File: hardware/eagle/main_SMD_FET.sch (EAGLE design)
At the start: 44 parts, among them IC1 R-78E3.3-1.0, IC2 INA186A1QDCKRQ1, IC3 ESP-12E/F, J4 1727078, Q1 IRFU3710ZPBF, Q2 IRFU3710ZPBF, Q3 IRFU3710ZPBF, Q4 IRFU3710ZPBF

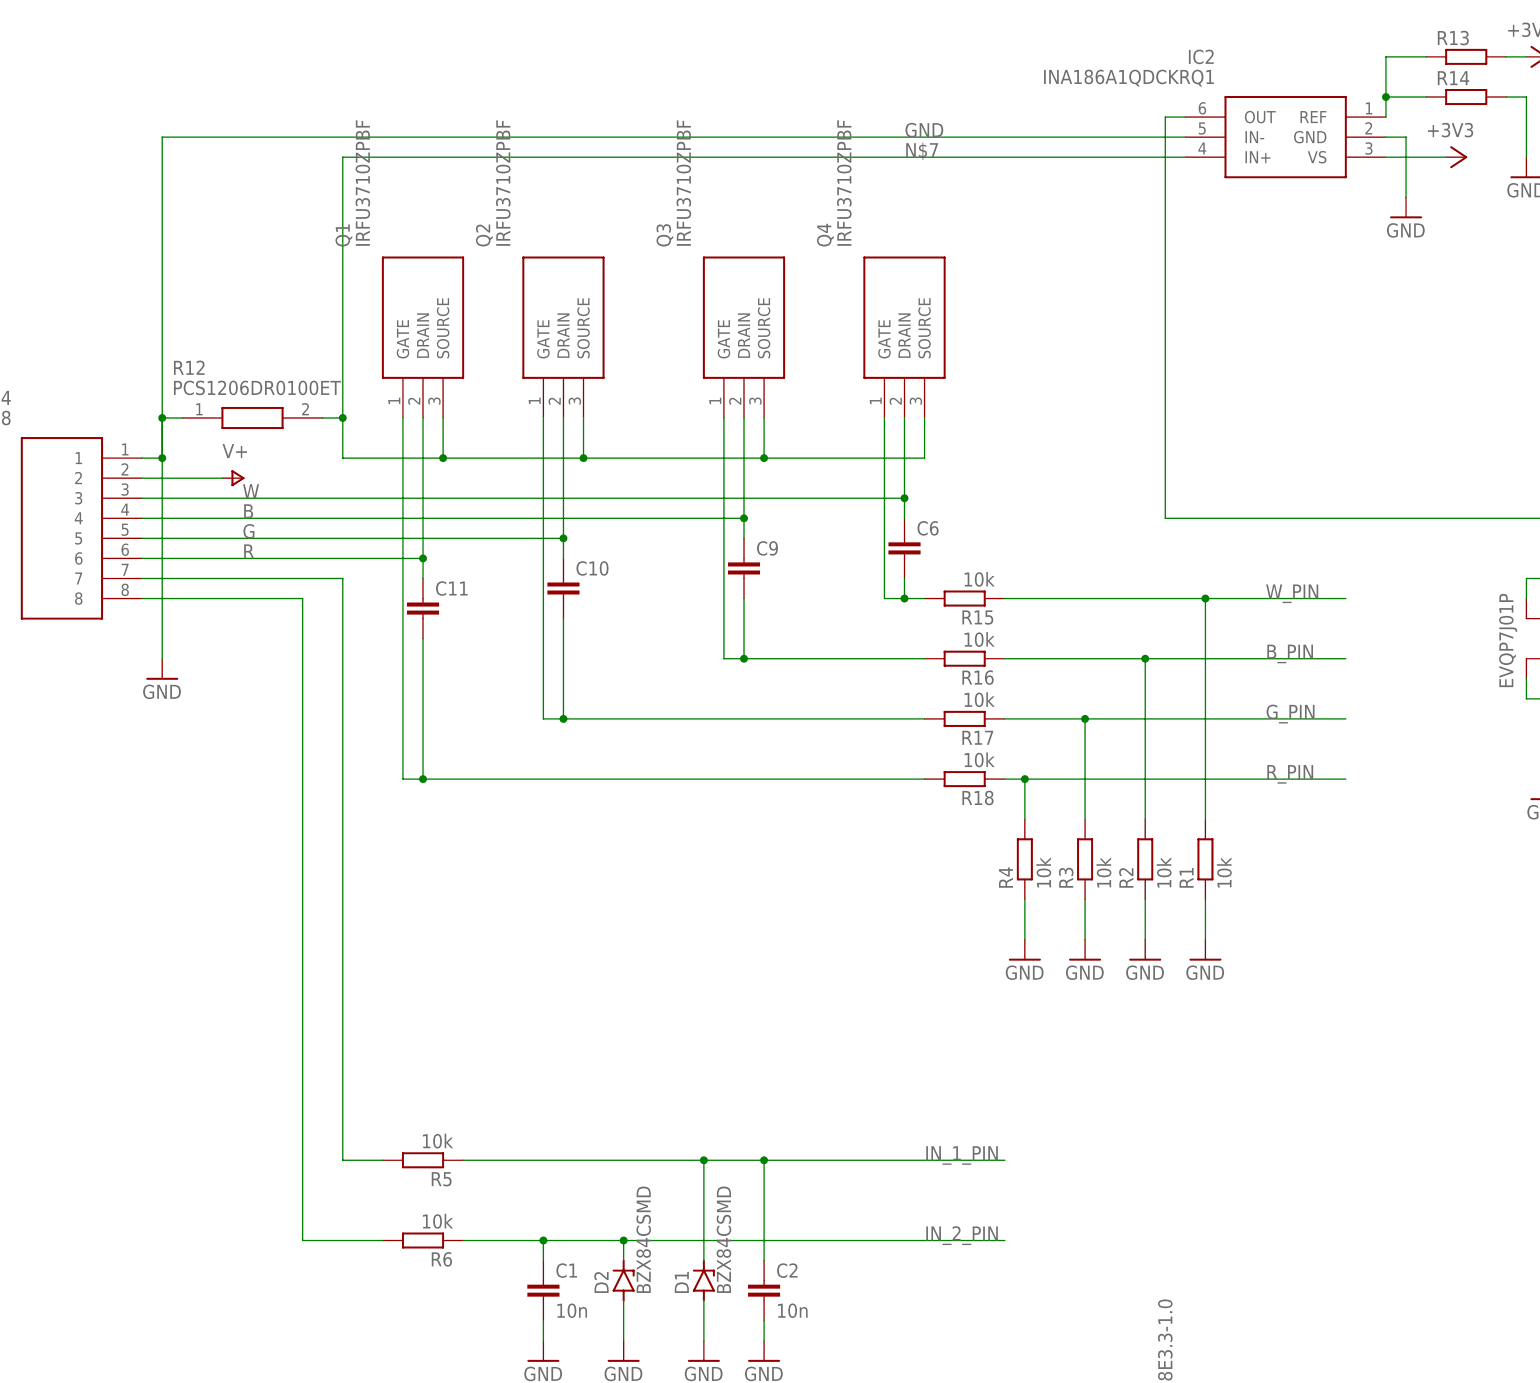
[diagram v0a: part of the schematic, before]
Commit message: initial
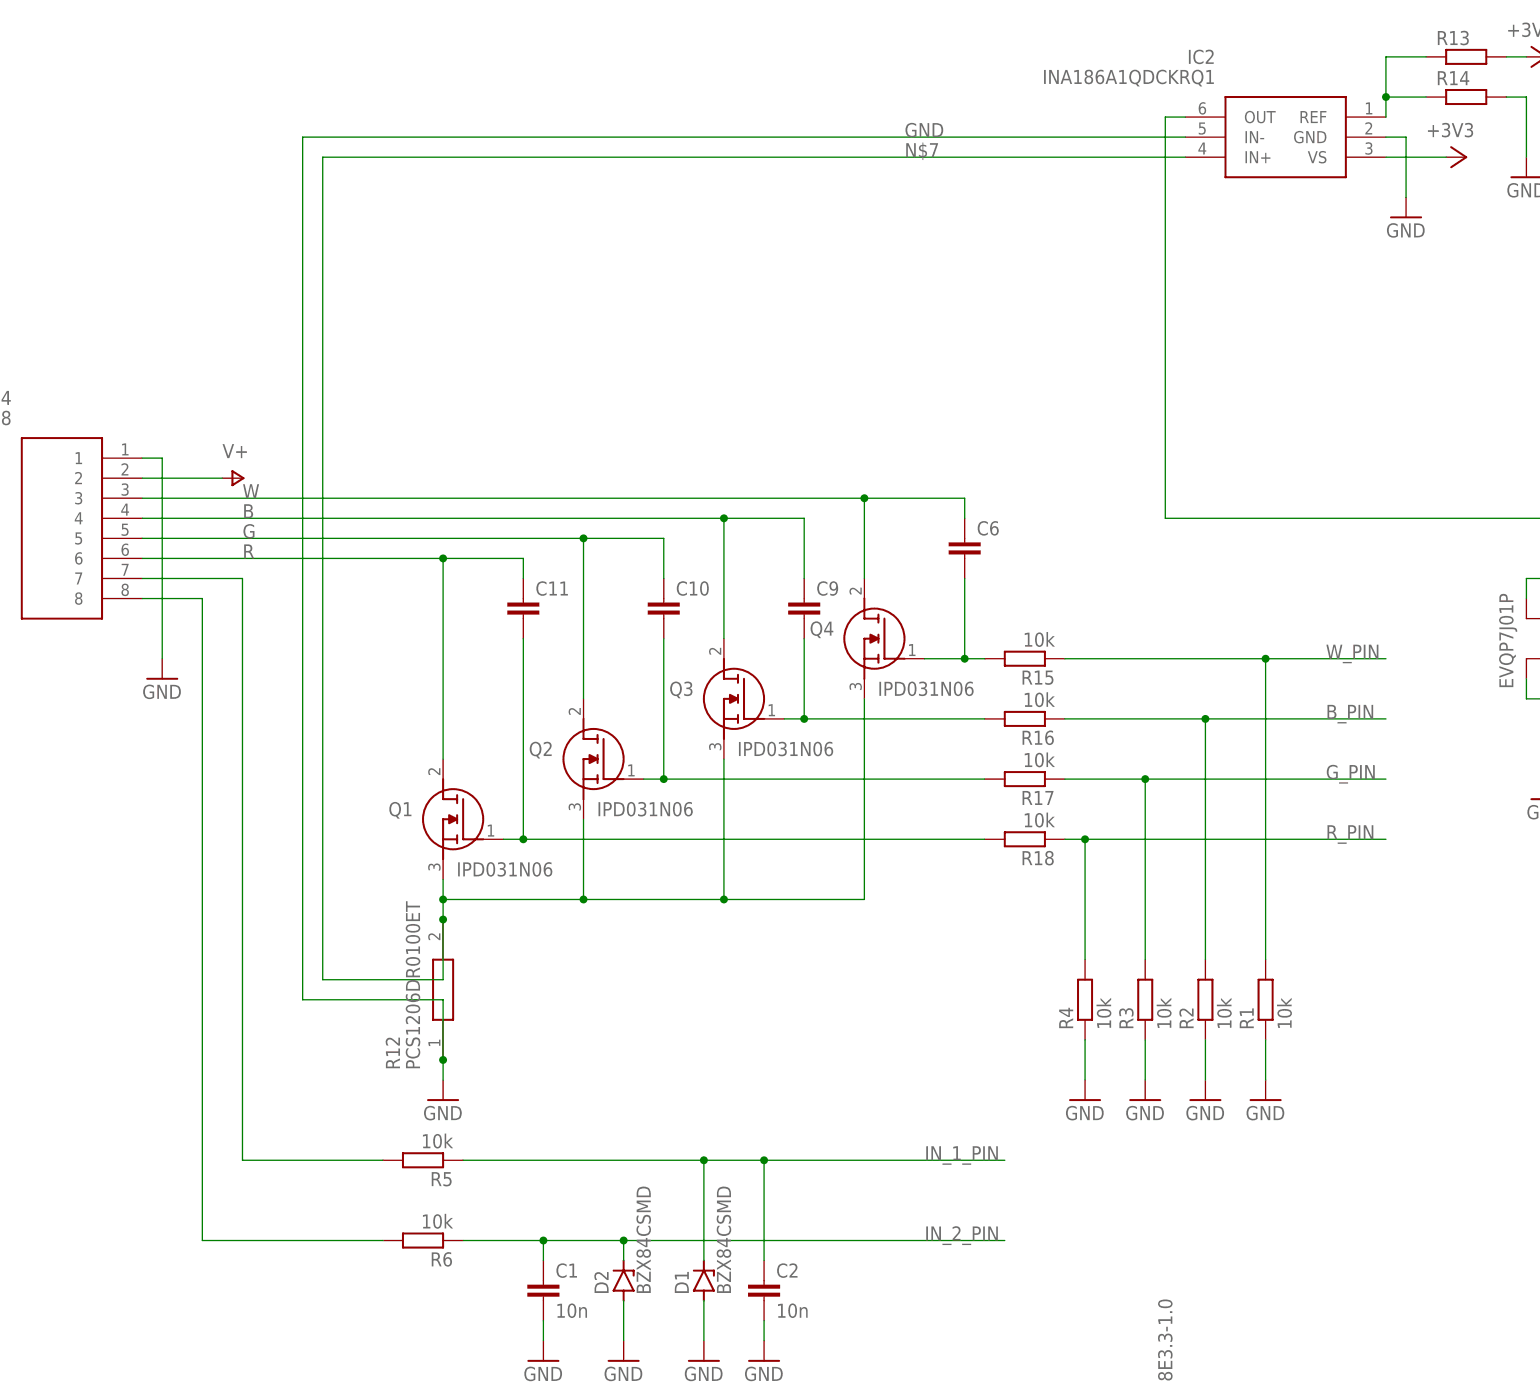
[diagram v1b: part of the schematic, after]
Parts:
- Q1, Q2, Q3, Q4: value IRFU3710ZPBF -> IPD031N06; device SamacSys_Parts:IRFU3710ZPBF -> SamacSys_Parts:IPD031N06L3GATMA1
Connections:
- net B: now also Q3.D; no longer Q3.DRAIN
- net G: now also Q2.D; no longer Q2.DRAIN
- net N$12: now also Q2.G; no longer Q2.GATE
- net N$14: now also Q3.G; no longer Q3.GATE
- net N$15: now also Q4.G; no longer Q4.GATE
- net N$2: now also Q1.G; no longer Q1.GATE
- net N$7: now also Q1.S, Q2.S, Q3.S, Q4.S; no longer Q1.SOURCE, Q2.SOURCE, Q3.SOURCE, Q4.SOURCE
- net R: now also Q1.D; no longer Q1.DRAIN
- net W: now also Q4.D; no longer Q4.DRAIN
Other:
- moved on the sheet: C10, C11, C6, C9, R1, R12, R15, R16, R17, R18, R2, R3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
